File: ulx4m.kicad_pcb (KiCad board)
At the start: 6 copper layers, 55.1 x 40 mm, 218 parts, among them IC1 VSC8530XMW-04, J1 DF40C-100DP-0.4V(51), J2 DF40C-100DP-0.4V(51), J3 JTAG, SW1 SW_Push, SW2 SW_Push, U1 LFE5U-85F-6BG381C, U10 IS25LP128F-JBLE, U2 AS4C256M16D3, U3 TLV62569DBV, U4 TLV62569DBV, U5 TLV62569DBV, U6 TLV62569DBV, Y1 FNETHE025

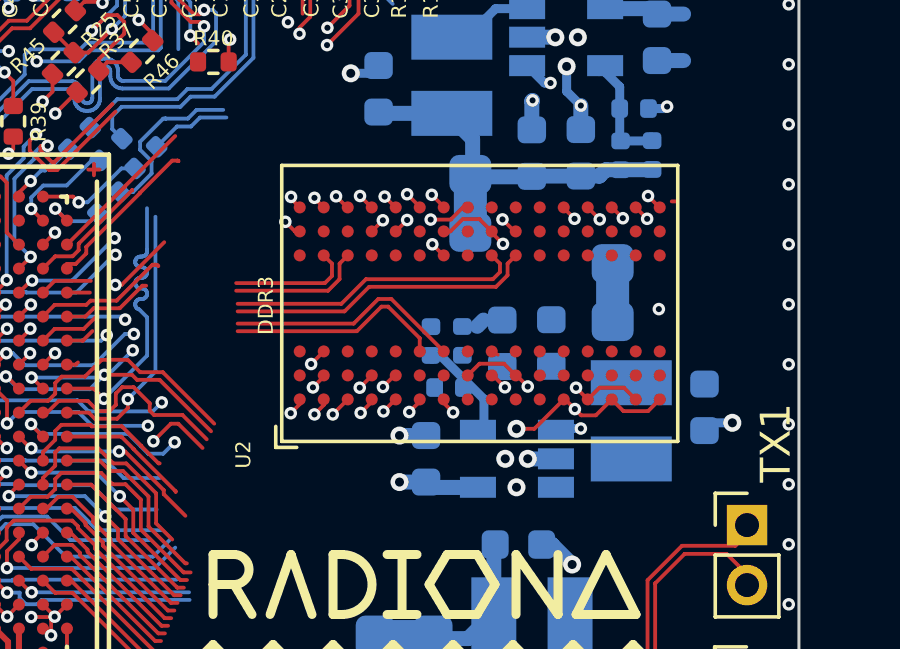
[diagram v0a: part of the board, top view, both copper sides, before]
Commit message: Rounting out DDR3
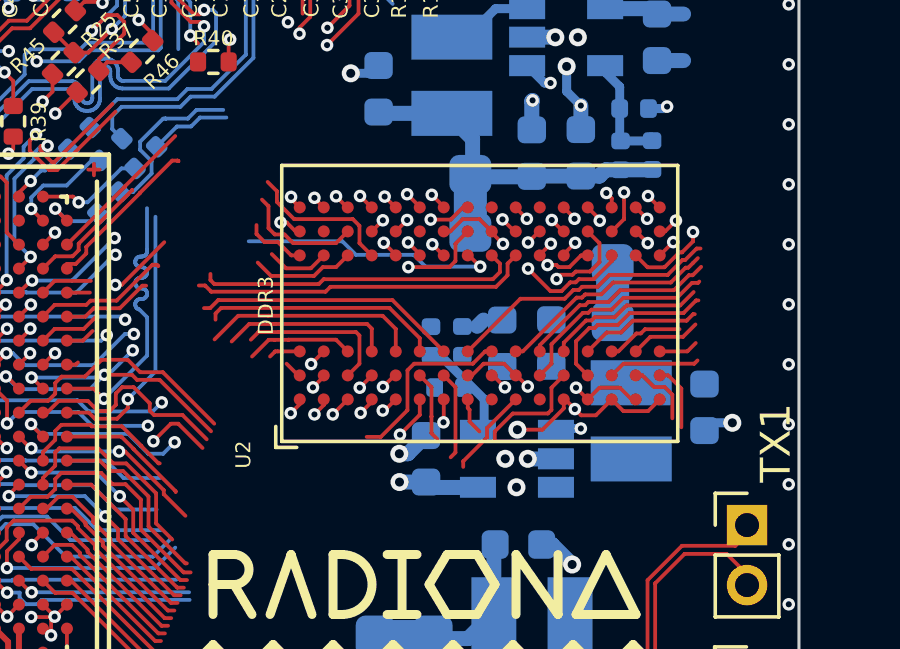
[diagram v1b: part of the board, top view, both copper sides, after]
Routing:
- net DDR3_DQ4: track 5.09 -> 14.3 mm
- net DDR3_DQ7: track 7.24 -> 15.9 mm, vias 1 -> 2
- net DDR3_CAS: track 8.83 -> 16.2 mm
- net DDR3_DQ0: track 6.91 -> 14.2 mm
- net DDR3_CS: track 7.82 -> 14.8 mm
- net DDR3_WE: track 7.50 -> 14.2 mm
- net DDR3_RAS: track 7.35 -> 13.5 mm
- net DDR3_A3: track 1.76 -> 7.70 mm
- net DDR3_DM1: track 0.40 -> 6.13 mm
- net DDR3_BA2: track 3.58 -> 8.90 mm
- net DDR3_DQ11: track 15.4 -> 20.6 mm
- net DDR3_DQ8: track 5.83 -> 10.9 mm
- net DDR3_A0: track 5.55 -> 9.63 mm
- net DDR3_DQ10: track 9.23 -> 13.3 mm
- net DDR3_BA0: track 8.38 -> 12.2 mm
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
